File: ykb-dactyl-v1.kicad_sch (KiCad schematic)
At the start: 1 part

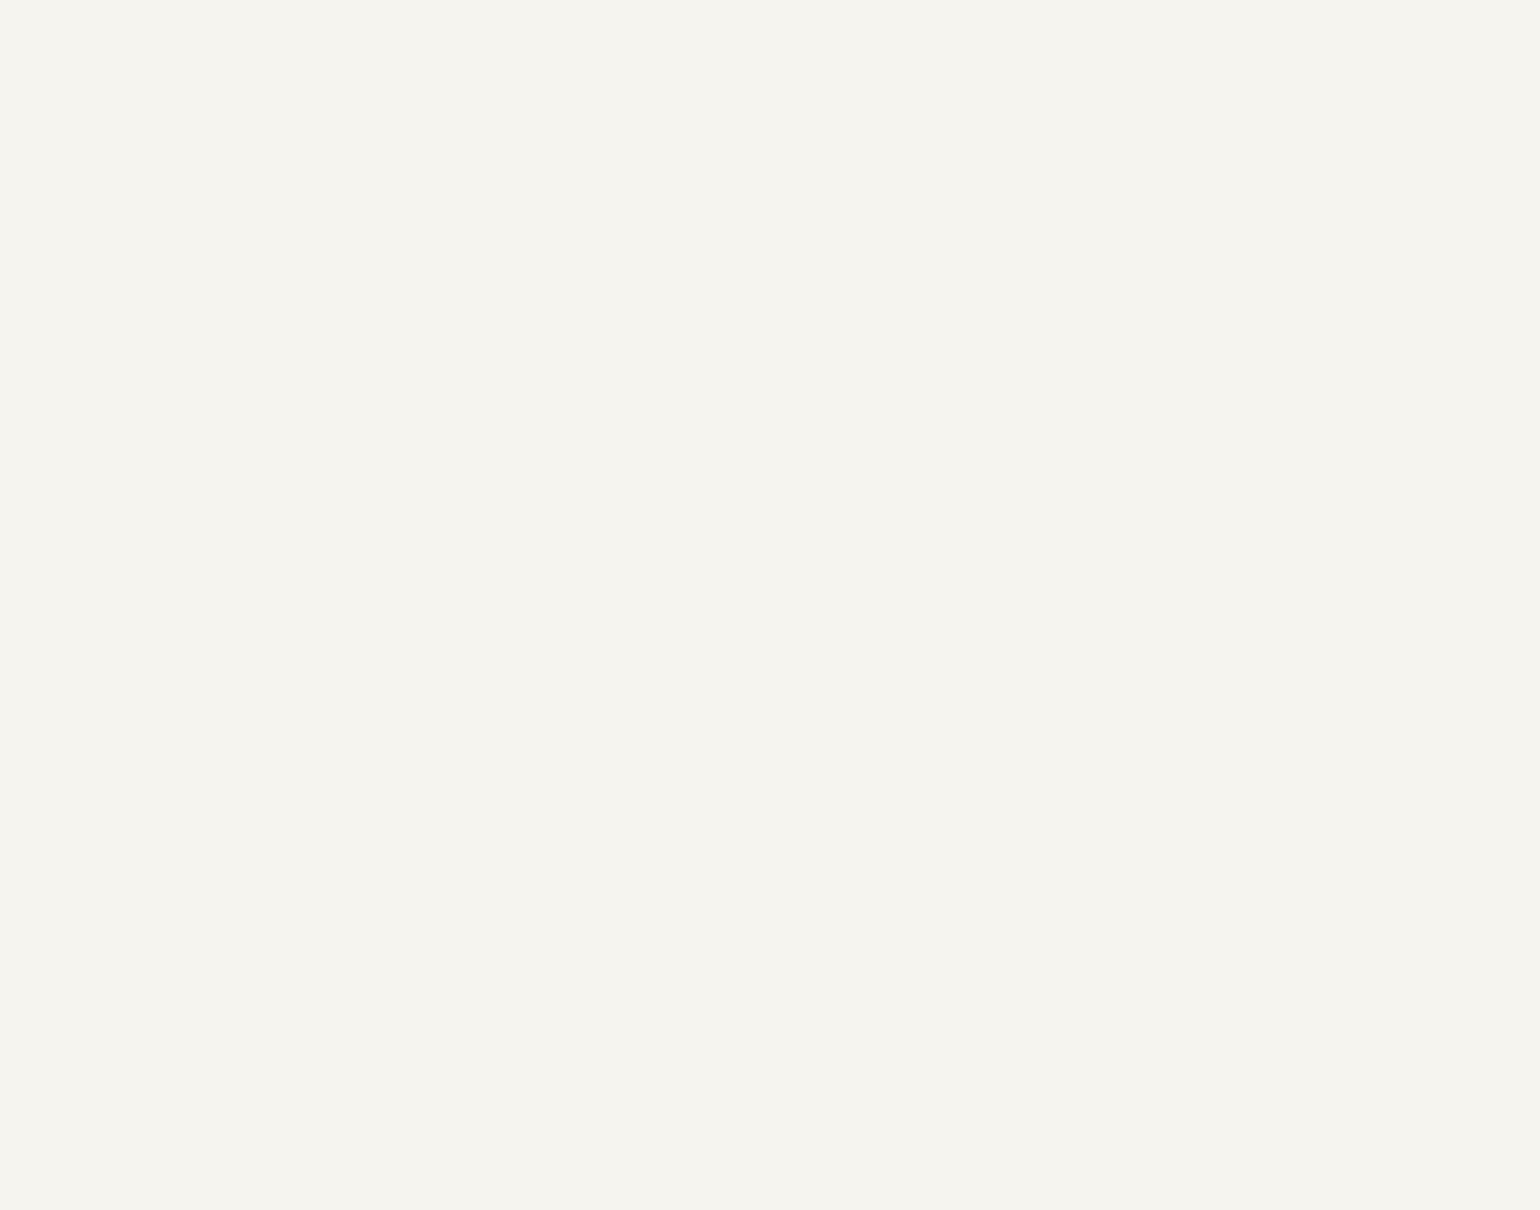
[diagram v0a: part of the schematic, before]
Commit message: Update
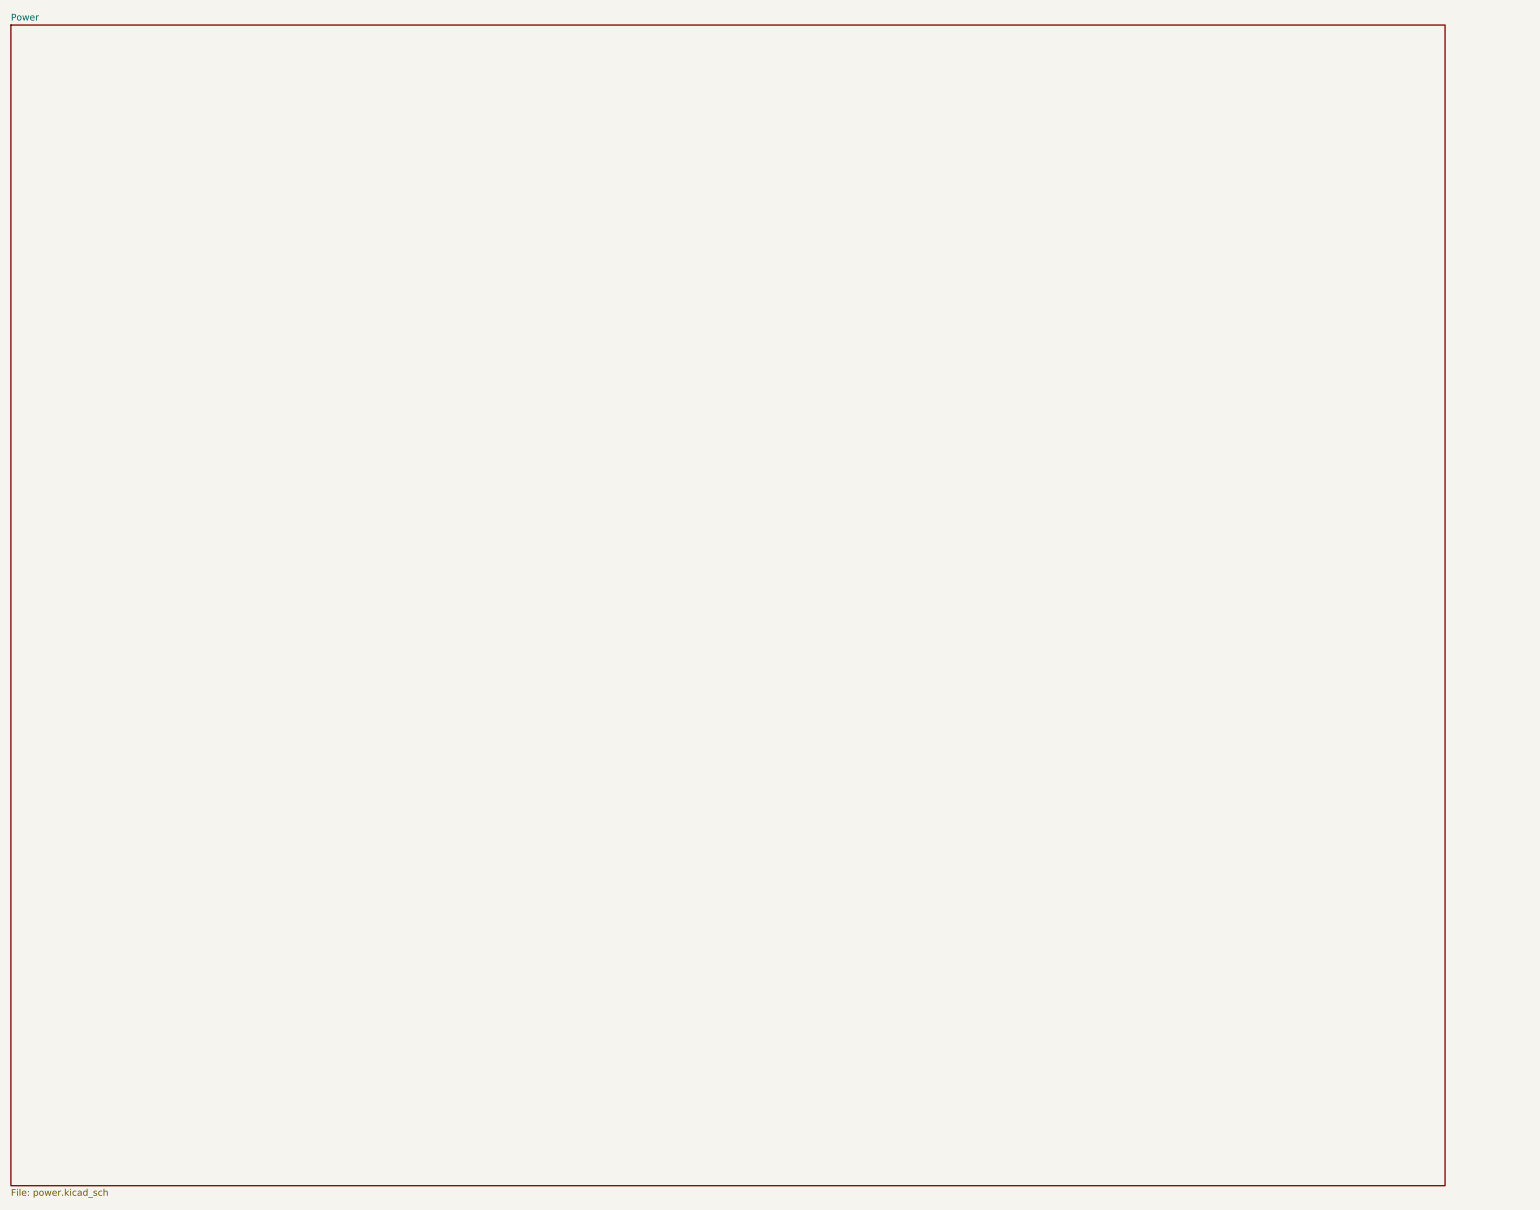
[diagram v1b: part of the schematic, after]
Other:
- added sheet Power (power.kicad_sch)
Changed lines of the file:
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@@
+		)
+	)
+	(sheet
+		(at -304.8 11.43)
+		(size 273.05 220.98)
+		(exclude_from_sim no)
+		(in_bom yes)
+		(on_board yes)
+		(dnp no)
+		(fields_autoplaced yes)
+		(stroke
+			(width 0.1524)
+			(type solid)
+		)
+		(fill
+			(color 0 0 0 0.0000)
+		)
+		(property "Sheetname" "Power"
+			(at -304.8 10.7184 0)
+			(effects
+				(font
+					(size 1.27 1.27)
+				)
+				(justify left bottom)
+			)
+		)
+		(property "Sheetfile" "power.kicad_sch"
+			(at -304.8 232.9946 0)
+			(effects
+				(font
+					(size 1.27 1.27)
+				)
+				(justify left top)
+			)
+		)
+		(instances
+			(project "ykb-dactyl-v1"
+				(path "/e14fa40b-de41-4d68-adfe-82a50bad5819"
+					(page "2")
+				)
+			)
 		)
 	)
